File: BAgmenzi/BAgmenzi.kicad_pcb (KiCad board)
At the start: 6 copper layers, 53.6 x 58.5 mm, 147 parts, among them IC1 TPL0501-100RSER, J1 Conn_01x07, J2 DF52-2S-0.8H(21), J3 USB3076-30-A, J4 connector for CMUT, J5 3220-10-0100-00, Q1 NX7002BKMBYL, U1 MSP430FR5043IRGCT, U10 PESD1USB30, U11 MAX77654BENV+T, U13 TPS7A2033DBVDQN, U2 AD8338ACPZ-R7, U3 OPA836IDBVT, U4 OPA836IDBVT, U7 LT3463AEDD#PBF, U8 TPS22916CYFPR, U9 MAXM86161EFD_T, X1 FY0800018, X2 ABS07-32.768KHZ-9-T, Y1 AWSCR-8.00CV-T

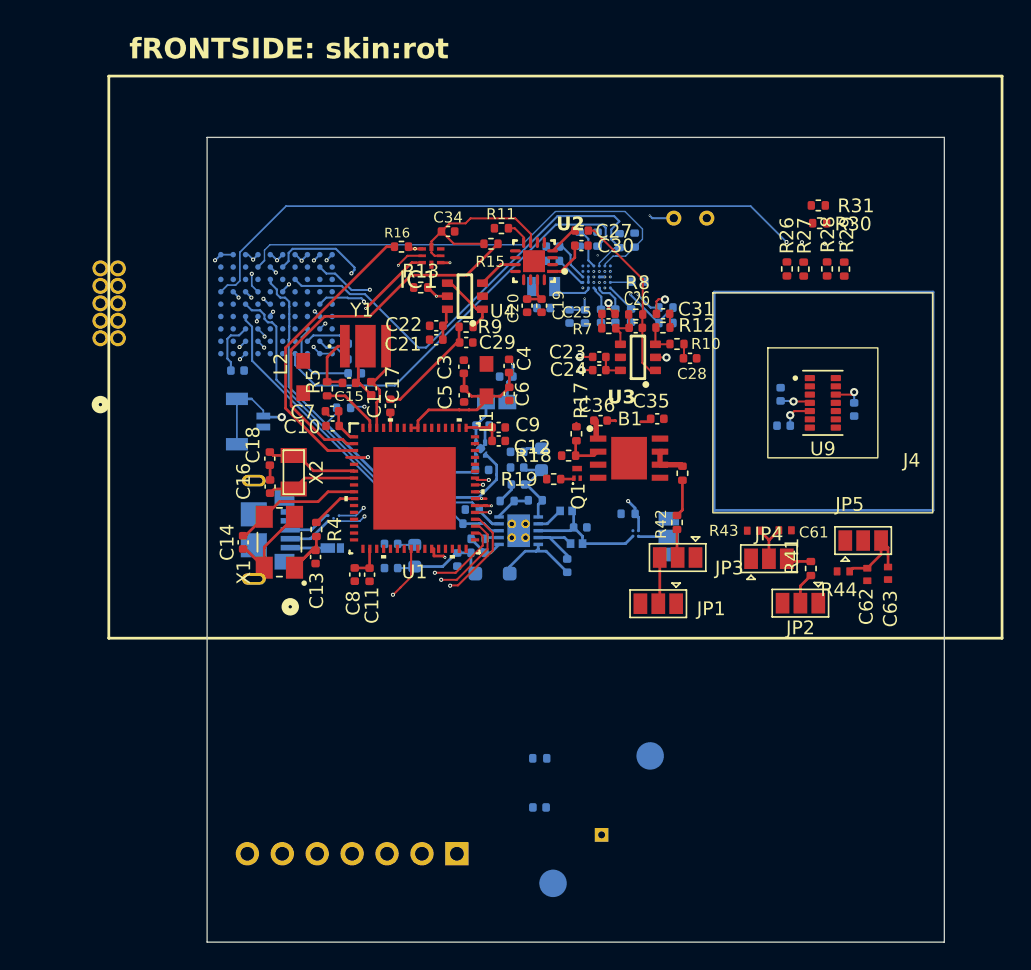
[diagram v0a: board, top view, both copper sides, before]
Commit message: powerplanes
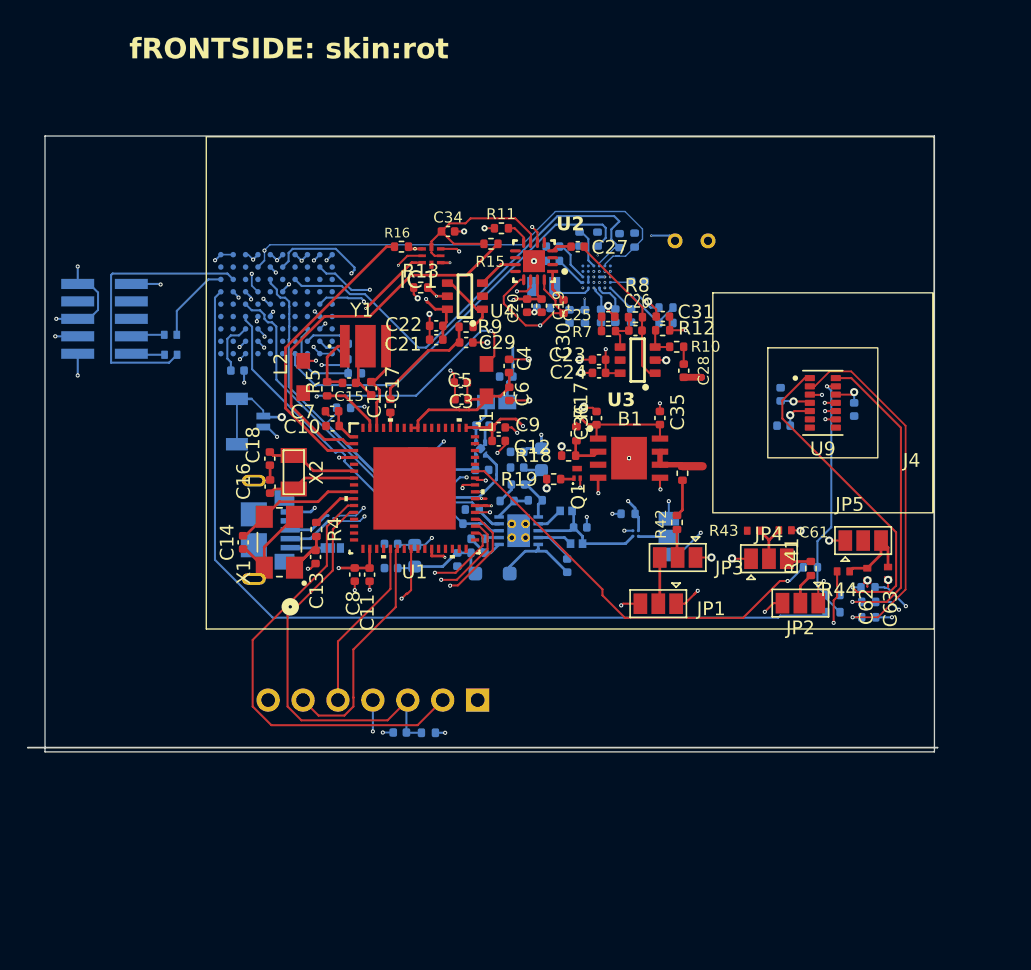
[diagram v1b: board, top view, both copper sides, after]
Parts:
- removed TP2: vga_vref, TestPoint:TestPoint_Pad_D2.0mm
- removed TP6: TestPoint, TestPoint:TestPoint_Pad_D2.0mm
- removed TP7: +V_hv_in, TestPoint:TestPoint_THTPad_1.0x1.0mm_Drill0.5mm
- added R45: 220, EEG_PcbLib:0402, B.Cu at (116.7, 104.9)
- added R46: 220, EEG_PcbLib:0402, B.Cu at (116.7, 103.5)
- J5: footprint EEG_PcbLib:CONN_3220-10-0100-00_CNC -> Connector_PinHeader_1.27mm:PinHeader_2x05_P1.27mm_Vertical_SMD
- R26, R27, R28, R29, R30, R31: moved to B.Cu
- moved R30 28.3 mm to (164.9, 123.7), turned to 180 degrees
- moved R31 26.3 mm to (163.2, 120.4), turned to 180 degrees
- moved R26 26.0 mm to (167.5, 124.0), turned to 180 degrees
- moved R28 24.4 mm to (167.5, 122.9), turned to 180 degrees
- moved R29 23.7 mm to (164.9, 122.4), turned to 180 degrees
- moved R27 23.6 mm to (167.4, 121.9), turned to 180 degrees
- moved C2 11.5 mm to (133.3, 132.4)
- moved J1 11.3 mm to (139.0, 130.1)
- moved R1 8.31 mm to (135.4, 132.4)
- moved C30 4.63 mm to (145.3, 101.4), turned to 90 degrees
- moved S1 1.65 mm to (155.8, 96.7)
- moved J5 1.44 mm to (111.9, 102.3), turned to 0 degrees
- moved C27 1.21 mm to (146.3, 97.1)
- moved C3 1.17 mm to (137.8, 107.0), turned to 180 degrees
- moved C28 1.01 mm to (154.0, 106.1), turned to 90 degrees
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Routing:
- net PPG_I2C.SCL: track 46.3 -> 93.4 mm
- net GND: track 43.8 -> 89.8 mm, vias 23 -> 67
- net DVDD_3.3: track 20.5 -> 56.1 mm, vias 1 -> 13
- net JTAG.TEST: track 0.00 -> 33.1 mm
- net SPARE_PIN: track 0.00 -> 30.1 mm, vias 0 -> 1
- net JTAG.RESET_N: track 0.00 -> 29.6 mm
- net PPG_INT: track 54.6 -> 81.1 mm
- net /RX/VGA_REF: track 1.01 -> 23.8 mm, vias 0 -> 2
- net SWDIO: track 0.00 -> 20.5 mm
- net PPG_GPIO: track 46.0 -> 66.0 mm, vias 1 -> 0
- net Net-(U9-GPIO): track 0.00 -> 18.4 mm, vias 0 -> 1
- net BSL.UART_RX: track 0.00 -> 17.2 mm
- net +HV: track 2.76 -> 16.4 mm, vias 0 -> 4
- net PPG_I2C.SDA: track 67.3 -> 80.1 mm
- net BSL.UART_TX: track 0.00 -> 12.6 mm
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- added copper zone on In1.Cu, net (none)
- added copper zone on In4.Cu, net (none)
- added copper zone on In2.Cu, net +HV
- added copper zone on In2.Cu, net -HV
- added copper zone on In3.Cu, net DVDD_3.3
- added copper zone on In2.Cu, net V_BAT
- added copper zone on In2.Cu, net V_LED
- added copper zone on In2.Cu, net V_RX
- added copper zone on In2.Cu, net V_SYS
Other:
- board size 53.6 x 58.5 mm -> 66.2 x 44.8 mm
